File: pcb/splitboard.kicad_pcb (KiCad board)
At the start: 2 copper layers, 222.9 x 95.2 mm, 150 parts, among them IC1 ATMEGA32U4-MU, J1 Conn_02x05_Counter_Clockwise, J2 Conn_droite, J3 Conn_On_Off, Q1 Q_NPN_BCE, Q2 Q_NPN_BCE, SW1 SW_Push_LED, SW10 SW_Push_LED, SW101 SPST_TACT-KMR2, SW11 SW_Push_LED, SW12 SW_Push_LED, SW13 SW_Push_LED, SW14 SW_Push_LED, SW15 SW_Push_LED, SW16 SW_Push_LED, SW17 SW_Push_LED, SW18 SW_Push_LED, SW19 SW_Push_LED, SW2 SW_Push_LED, SW20 SW_Push_LED, SW21 SW_Push_LED, SW22 SW_Push_LED, SW23 SW_Push_LED, SW24 SW_Push_LED, SW25 SW_Push_LED, SW26 SW_Push_LED, SW27 SW_Push_LED, SW28 SW_Push_LED, SW29 SW_Push_LED, SW3 SW_Push_LED, SW30 SW_Push_LED, SW31 SW_Push_LED, SW32 SW_Push_LED, SW33 SW_Push_LED, SW34 SW_Push_LED, SW35 SW_Push_LED, SW36 SW_Push_LED, SW37 SW_Push_LED, SW38 SW_Push_LED, SW39 SW_Push_LED, SW40 SW_Push_LED, SW41 SW_Push_LED, SW42 SW_Push_LED, SW43 SW_Push_LED, SW44 SW_Push_LED, SW45 SW_Push_LED, SW46 SW_Push_LED, SW47 SW_Push_LED, SW5 SW_Push_LED, SW50 Rotary_Encoder, SW6 SW_Push_LED, SW7 SW_Push_LED, SW8 SW_Push_LED, SW9 SW_Push_LED, U1 TCA9555DBR, U2 TCA9555DBR, U3 MCP73831T-2ACI/OT, U4 SPX3819-3.3, U5 MBT40, X3 microUSB, Y1 8MHz

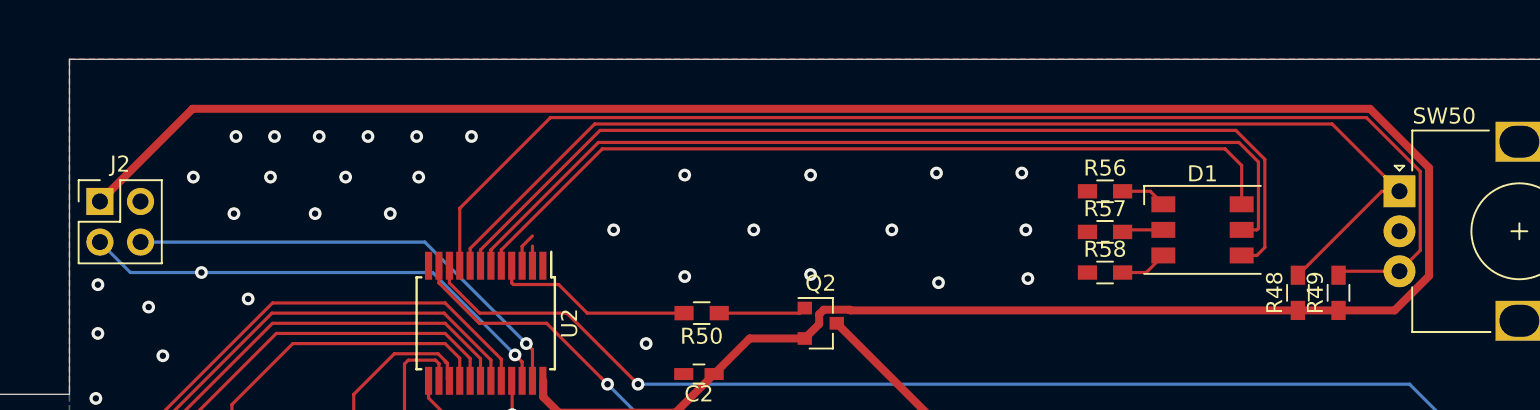
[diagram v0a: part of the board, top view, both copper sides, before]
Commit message: check wires
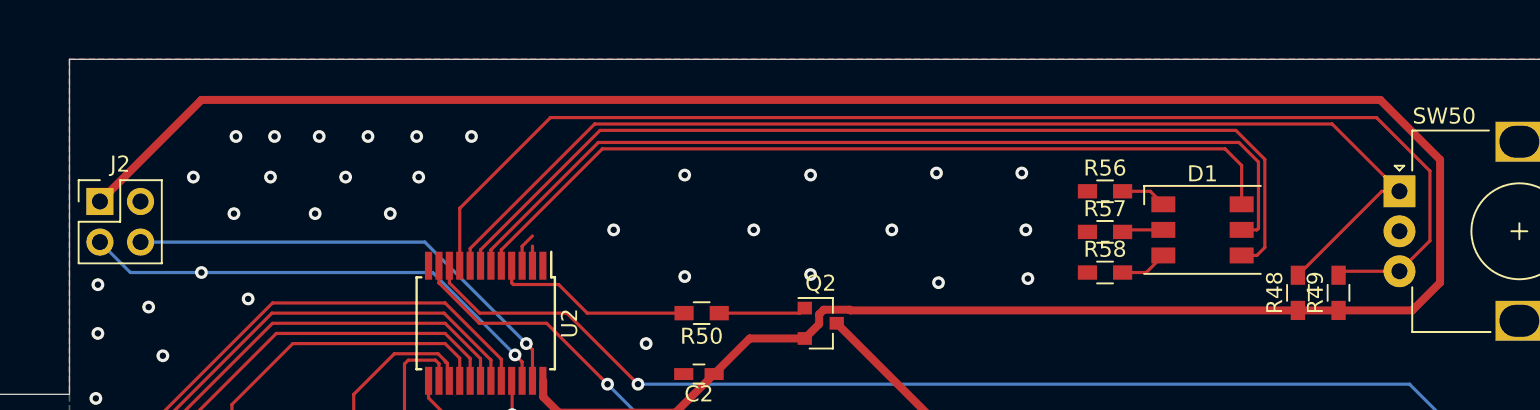
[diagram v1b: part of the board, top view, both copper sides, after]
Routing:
- net vcc1: track 154.6 -> 157.0 mm
- net Net-(R49-Pad2): track 78.1 -> 79.0 mm
